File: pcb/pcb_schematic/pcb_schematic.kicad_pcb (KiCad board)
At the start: 4 copper layers, 30.2 x 47.8 mm, 33 parts, among them J1 Conn_ST_STDC14, J3 Conn_02x02_Odd_Even, J4 USB_B_Micro, Q1 MMBT3904, Q2 MMBT3904, Q3 MMBT3904, U1 STM32G031K8Tx, U2 NCP1117-3.3_SOT223, U4 SSD1306 128 x 64 OLED (0x3C), U5 TCS34725 (0x29), Y1 Crystal

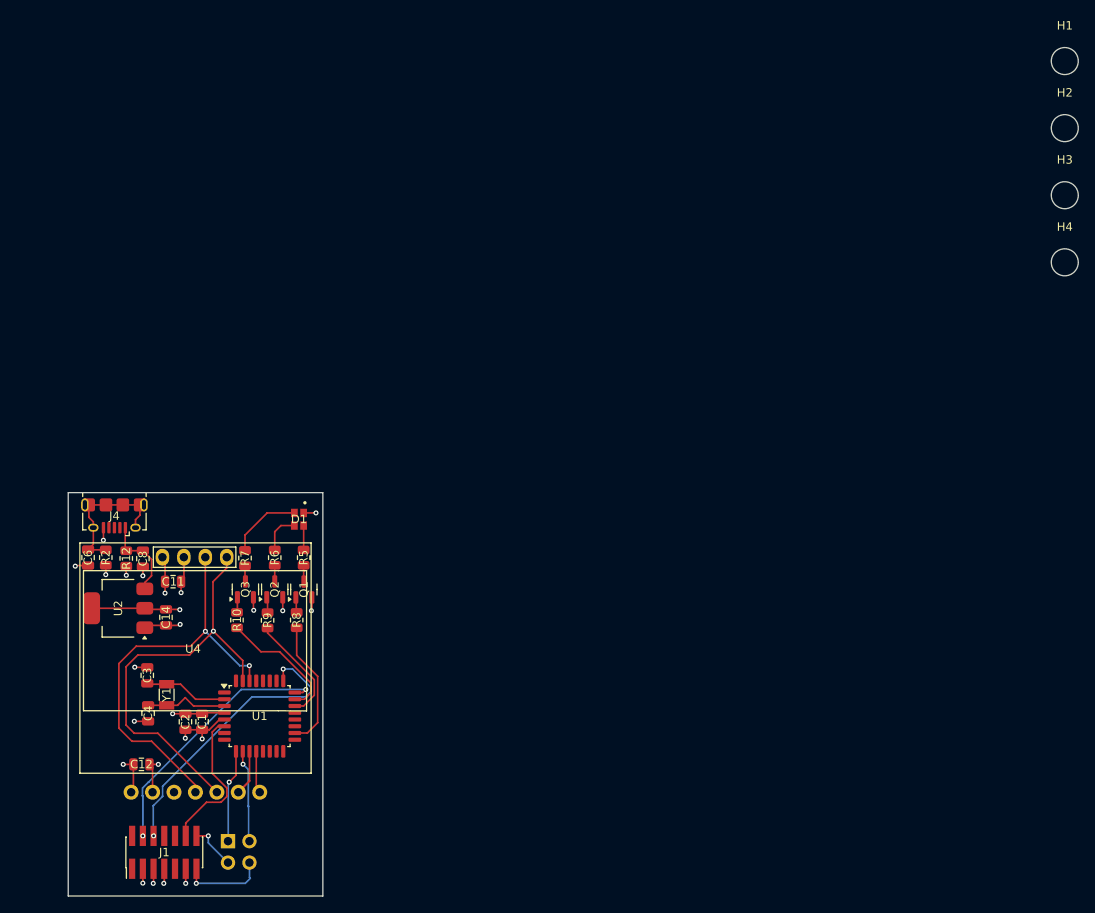
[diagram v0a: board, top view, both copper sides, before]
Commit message: before i change many thing
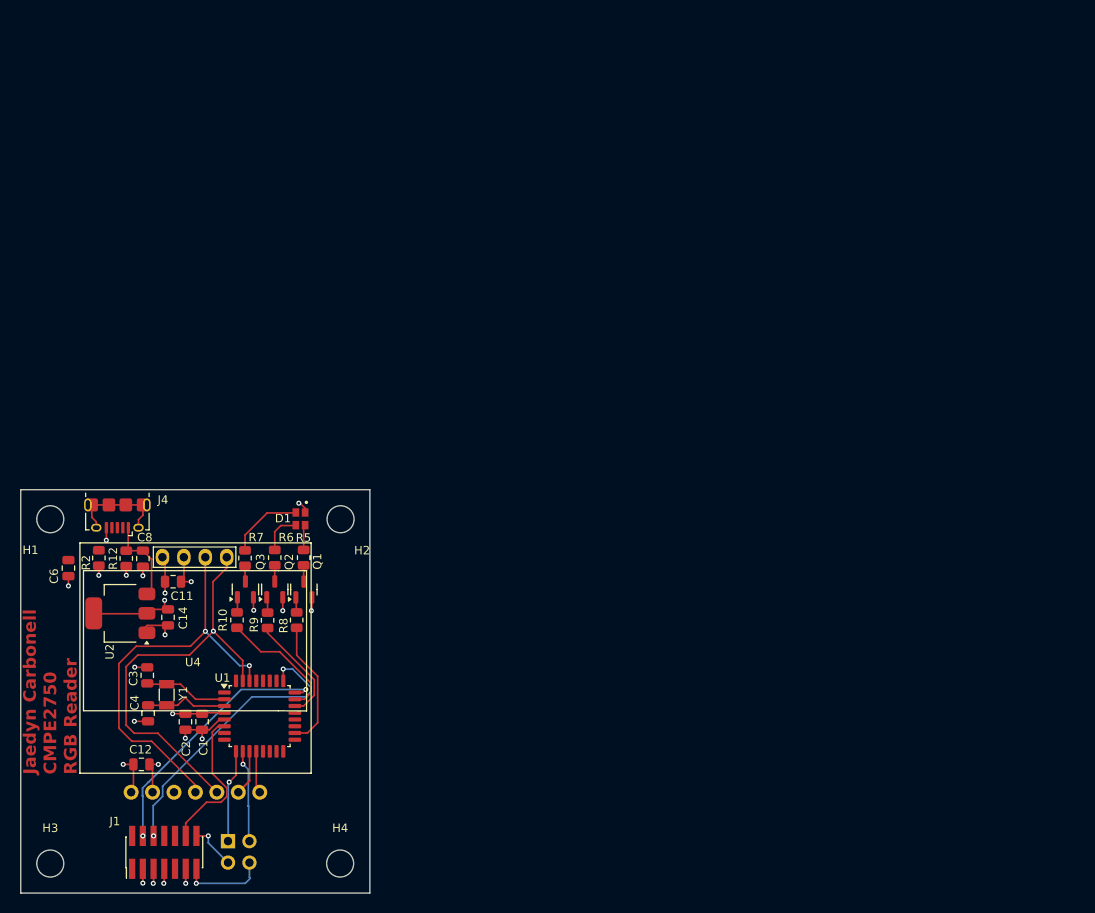
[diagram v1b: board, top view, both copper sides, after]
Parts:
- moved H3 144.0 mm to (154.5, 115.5)
- moved H1 131.9 mm to (154.5, 74.7)
- moved H4 111.6 mm to (188.8, 115.5)
- moved H2 97.5 mm to (188.9, 74.7)
- moved C6 2.64 mm to (156.7, 80.4)
- moved R2 0.83 mm to (160.2, 79.2)
- moved U2 0.65 mm to (162.8, 85.8)
- moved J4 0.35 mm to (162.4, 74.2)
- moved C14 0.24 mm to (168.4, 86.3)
- moved D1 0.18 mm to (184.2, 74.6)
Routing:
- net Net-(J4-Shield): track 17.6 -> 12.3 mm
- net GND: track 40.4 -> 39.4 mm
- net +3.3V: track 28.6 -> 28.1 mm
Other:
- board size 30.2 x 47.8 mm -> 41.4 x 47.8 mm
- board text added: "Jaedyn Carbonell CMPE2750 RGB Reader"
